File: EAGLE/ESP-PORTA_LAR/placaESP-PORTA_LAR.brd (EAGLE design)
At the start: 53.3 x 42.9 mm, 21 parts

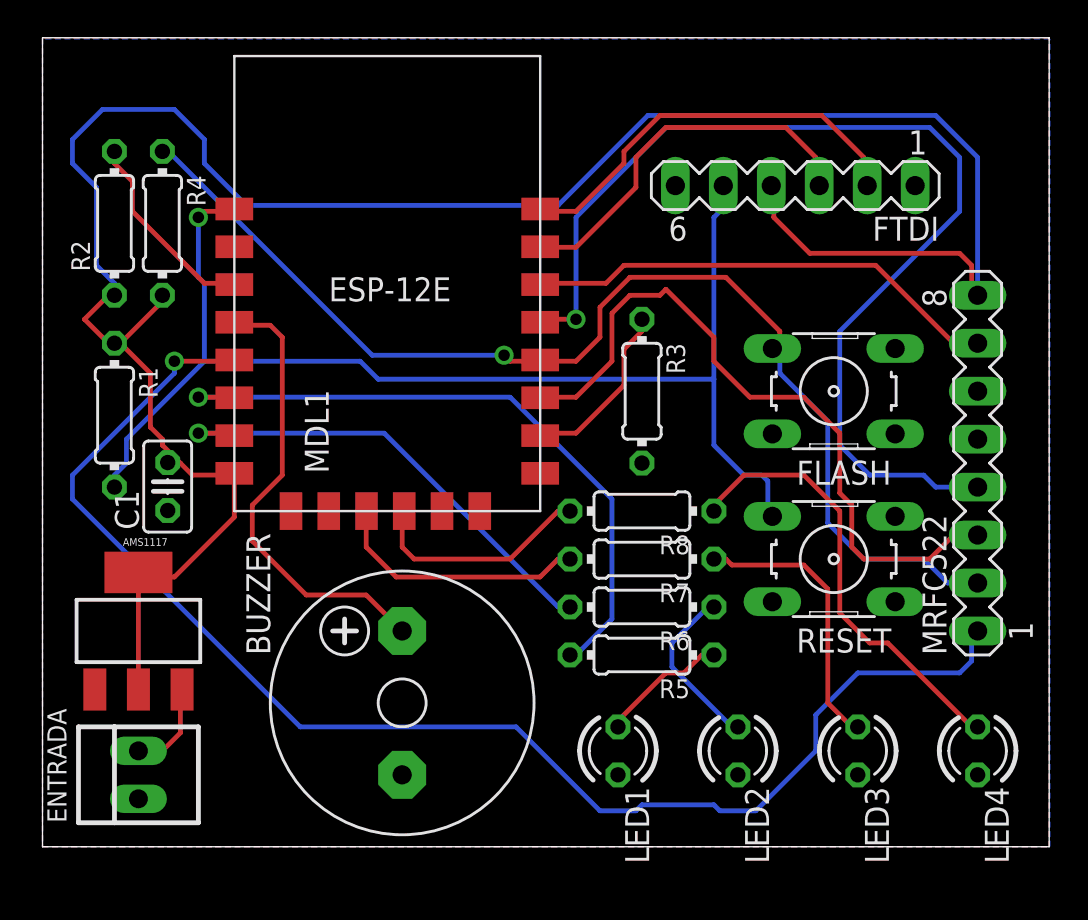
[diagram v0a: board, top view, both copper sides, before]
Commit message: Correções na placa da porta
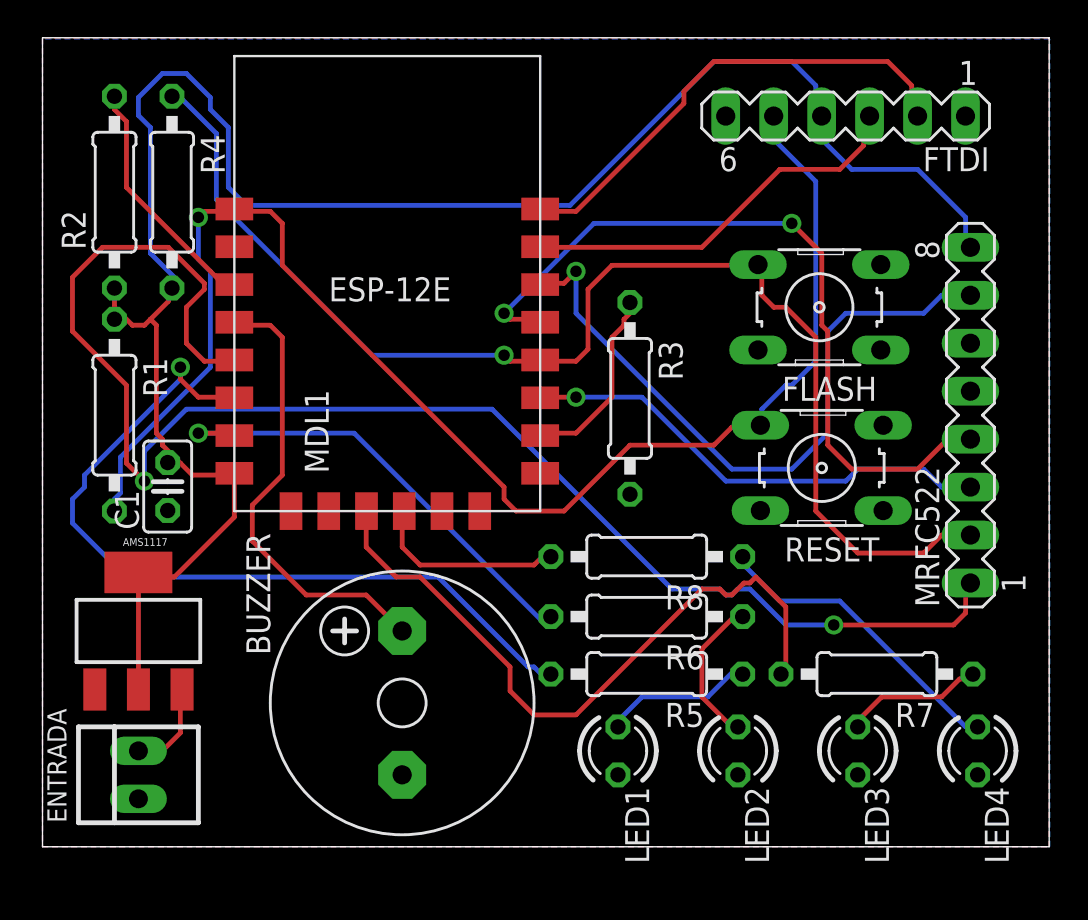
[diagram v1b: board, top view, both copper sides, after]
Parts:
- R1, R2, R3, R4, R5, R6, R7, R8: device resistor:0204/7 -> resistor:0207/10
- moved R7 13.9 mm to (44.2, 9.14)
- moved RESET 4.87 mm to (41.3, 20.1)
- moved FTDI 4.55 mm to (42.5, 38.7)
- moved FLASH 4.51 mm to (41.1, 28.6)
- moved MRFC522 2.57 mm to (49.1, 22.9)
- moved R8 2.43 mm to (32.0, 15.4)
- moved R4 1.73 mm to (6.86, 34.7)
- moved R2 1.65 mm to (3.81, 34.7)
- moved R5 1.05 mm to (32.0, 9.14)
- moved R3 0.74 mm to (31.1, 23.7)
- moved R6 0.57 mm to (32.0, 12.2)
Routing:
- net LED3: track 13.8 -> 36.3 mm
- net VCC: track 120.2 -> 104.1 mm
- net MISO: track 56.4 -> 40.7 mm, vias 1 -> 2
- net MOSI: track 37.4 -> 25.3 mm, vias 0 -> 1
- net CTS: track 65.5 -> 76.7 mm
- net RST: track 25.3 -> 35.7 mm, vias 0 -> 1
- net LED1: track 35.4 -> 43.4 mm
- net N$7: track 14.8 -> 7.53 mm
- net N$8: track 23.6 -> 16.4 mm
- net SDA: track 73.6 -> 80.5 mm, vias 1 -> 2
- net SCK: track 62.1 -> 67.2 mm
- net RXI: track 22.1 -> 25.8 mm
- net N$3: track 10.6 -> 13.0 mm
- net LED4: track 12.2 -> 10.6 mm
- net N$5: track 6.84 -> 8.39 mm
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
